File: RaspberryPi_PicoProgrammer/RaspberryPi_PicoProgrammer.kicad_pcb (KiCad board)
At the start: 2 copper layers, 20.2 x 55.2 mm, 7 parts, among them J1 Conn_02x05_Odd_Even, J2 Conn_01x03_Male, J3 Conn_02x03_Odd_Even, J4 BM03B-SRSS-TBLFSN, J5 Raspberry_Pi_2_3

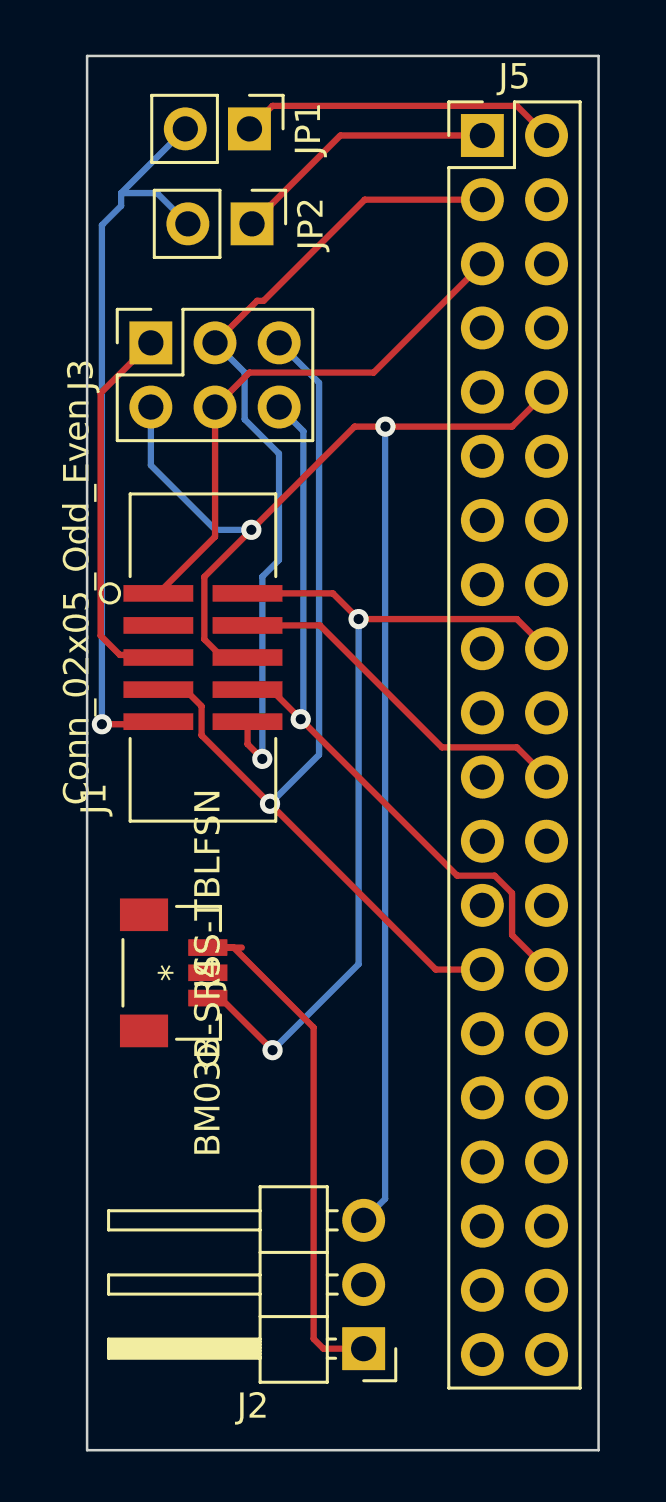
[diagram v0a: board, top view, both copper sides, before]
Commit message: board sent out
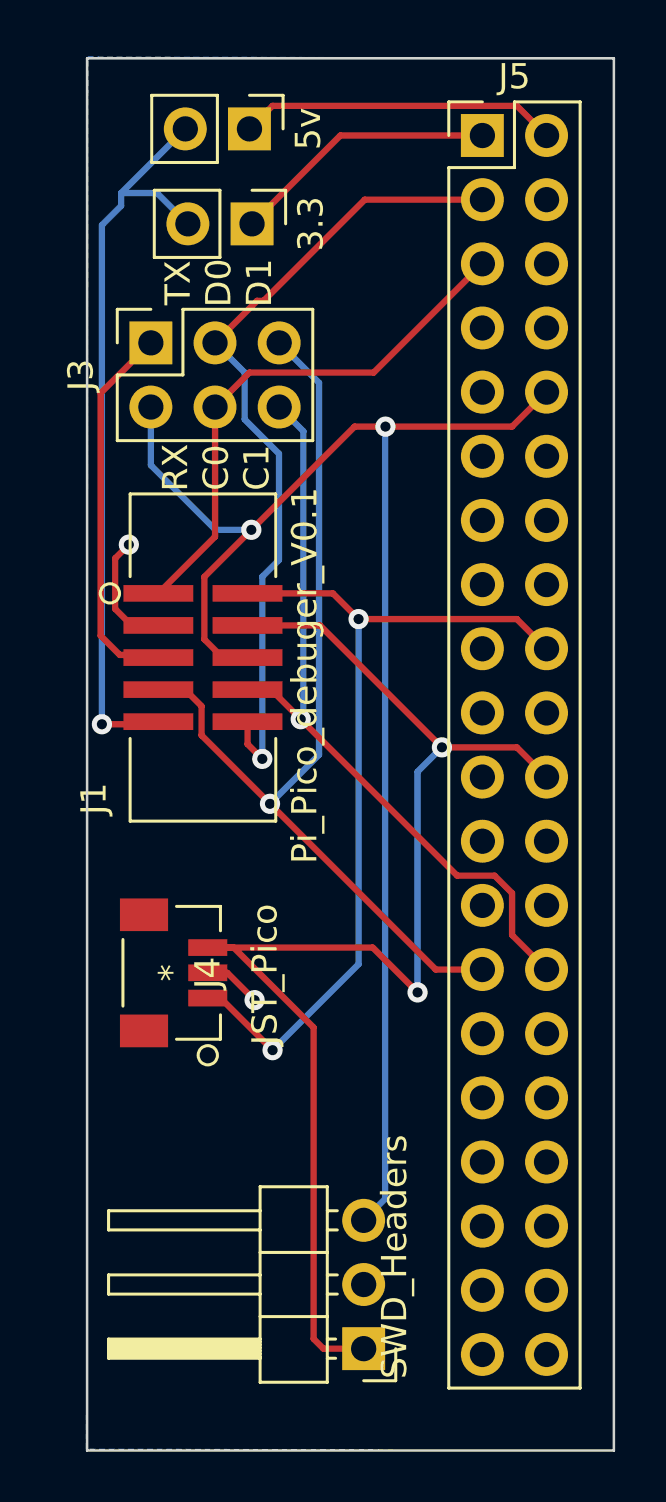
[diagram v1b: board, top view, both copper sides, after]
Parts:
- J1: value Conn_02x05_Odd_Even -> Pi_Pico_debuger_V0.1
- J3: value Conn_02x03_Odd_Even -> Conn_Extra
- J4: value BM03B-SRSS-TBLFSN -> JST_Pico
- renumbered JP2 to 3.3, JP1 to 5v, J2 to SWD_Headers
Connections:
- J5 pad 14: unconnected-(J5-Pad14) -> GND
- J5 pad 20: unconnected-(J5-Pad20) -> GND
- J5 pad 25: unconnected-(J5-Pad25) -> GND
- J5 pad 30: unconnected-(J5-Pad30) -> GND
- J5 pad 34: unconnected-(J5-Pad34) -> GND
- J5 pad 39: unconnected-(J5-Pad39) -> GND
- J5 pad 6: unconnected-(J5-Pad6) -> GND
- J5 pad 9: unconnected-(J5-Pad9) -> GND
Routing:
- net /SWDCLK: track 35.6 -> 53.4 mm, vias 0 -> 2
- net GND: track 0.00 -> 7.05 mm, vias 0 -> 2
- added copper zone on B.Cu, net GND
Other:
- board size 20.2 x 55.2 mm -> 20.9 x 55.1 mm
- board text added: "RX C0 C1"
- board text added: "TX D0 D1"
